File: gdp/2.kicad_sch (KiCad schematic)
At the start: 9 parts, among them IC1 74LS85, IC17 MK3881, IC7 PAL16L8

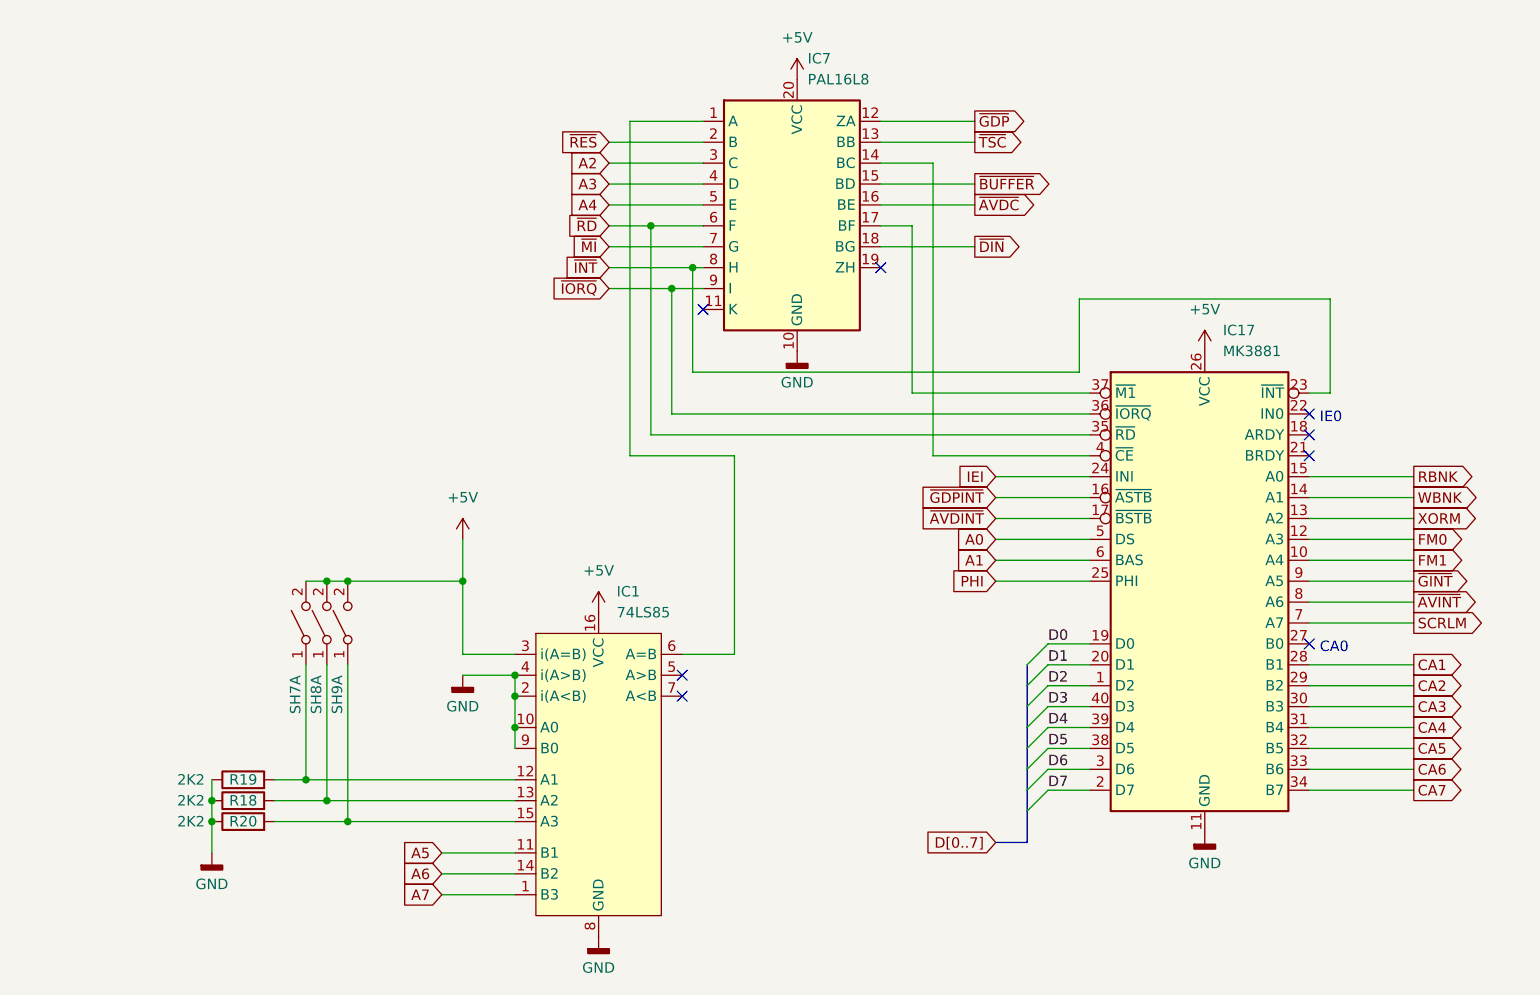
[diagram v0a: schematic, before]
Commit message: Adds Sheet 5
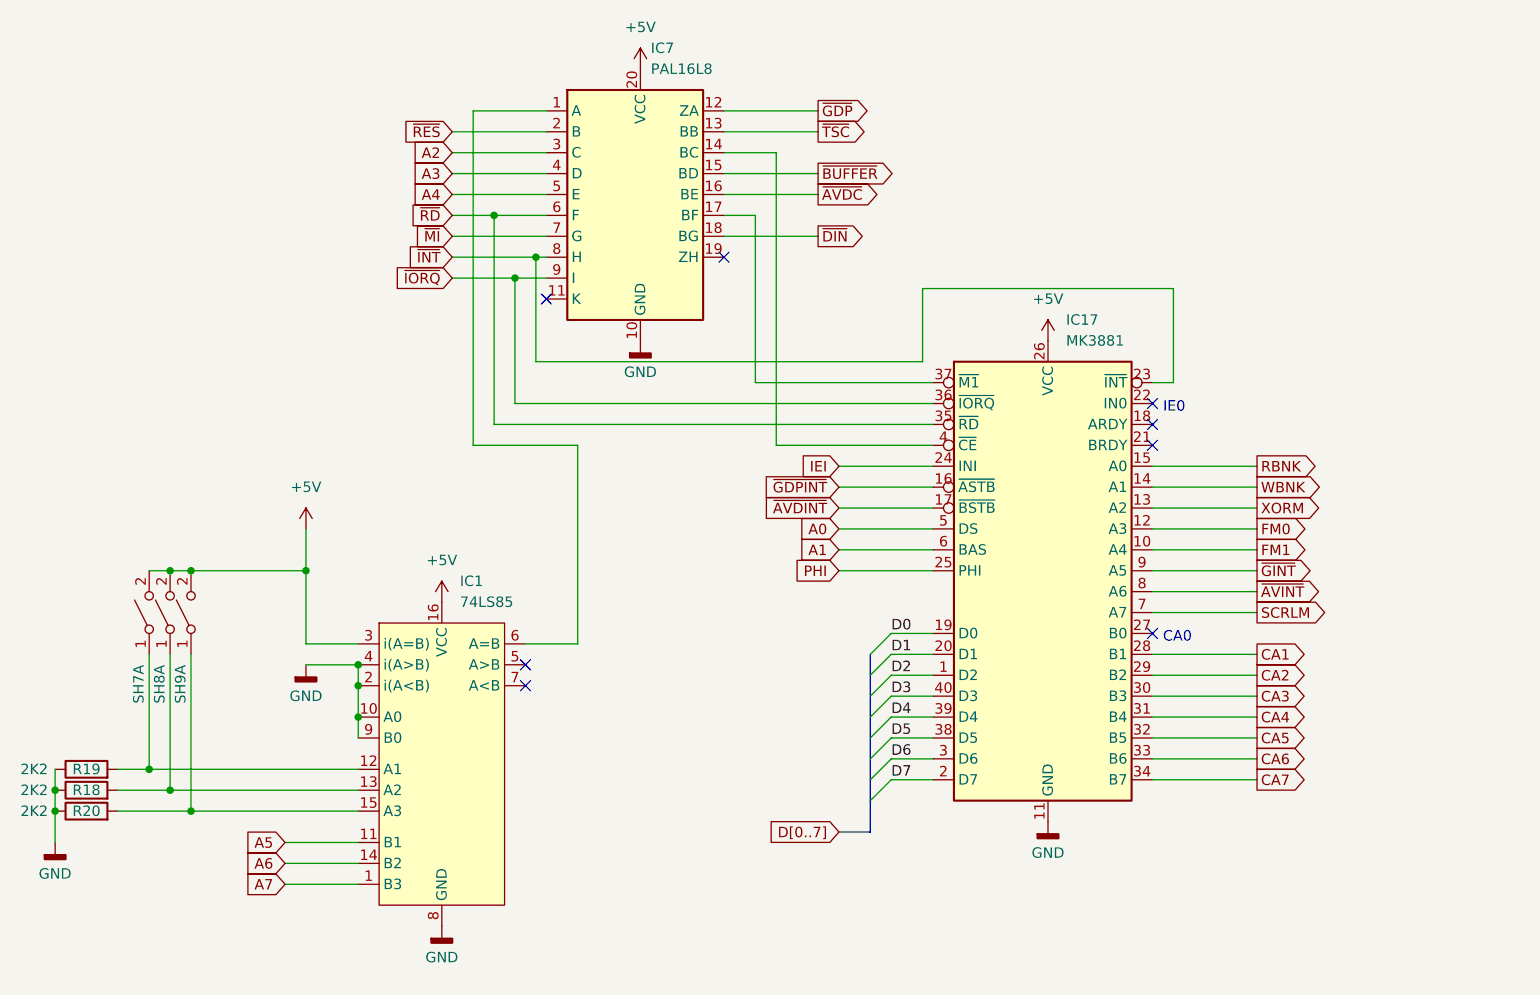
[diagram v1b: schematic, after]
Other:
- title: PARTNER GDP -> PARTNER GDP: ADRESIRANJE + PIO
- moved on the sheet: IC1, IC17, IC7, R18, R19, R20, SH7A, SH8A, SH9A
